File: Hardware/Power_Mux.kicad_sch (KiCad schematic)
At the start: 6 parts, among them U5 TPS2117DRLR

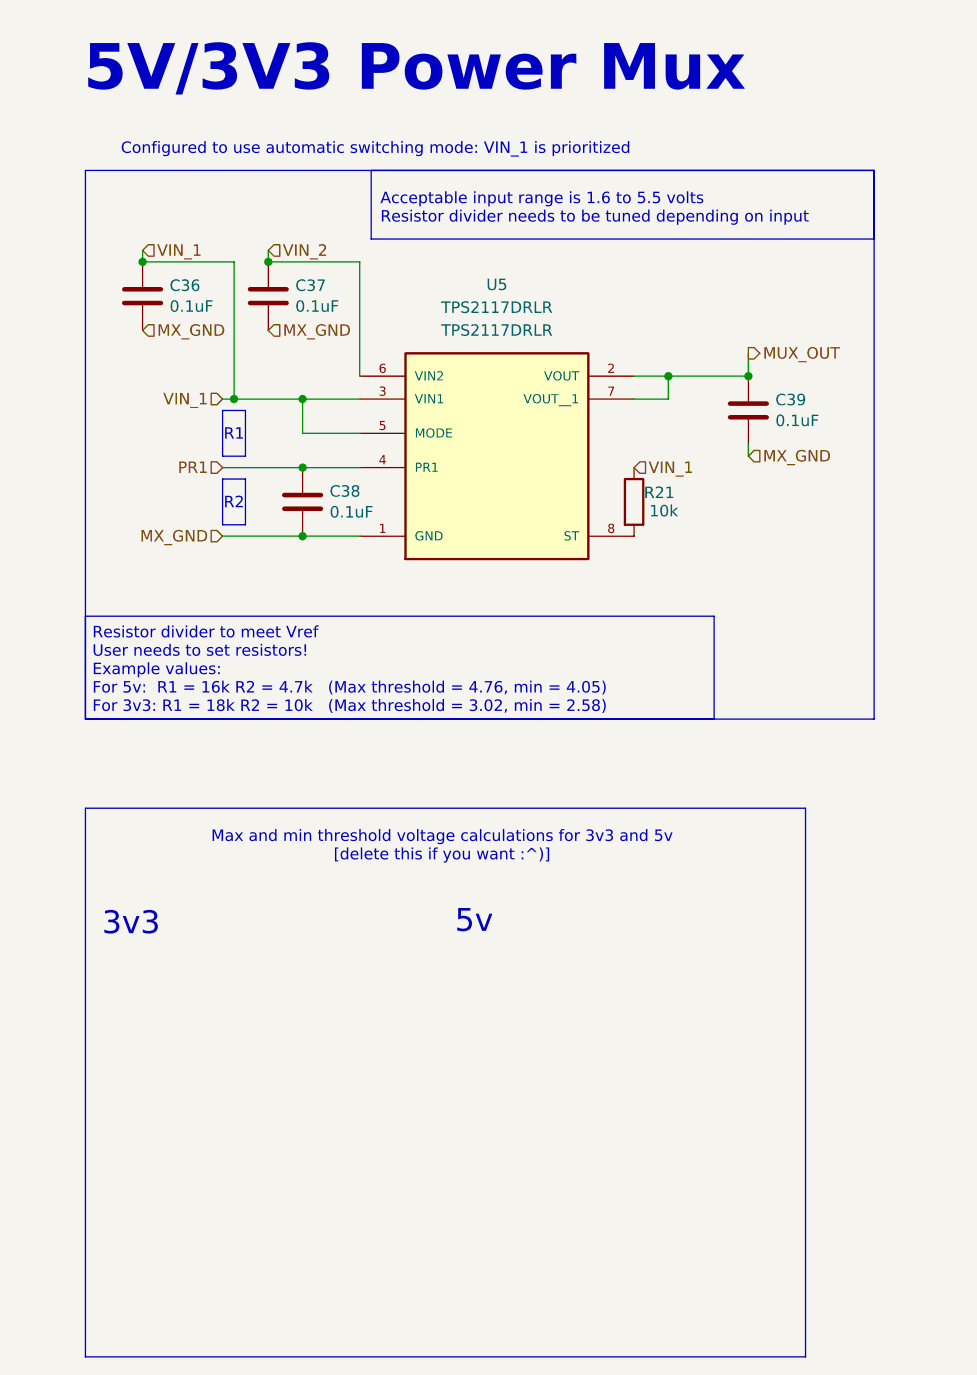
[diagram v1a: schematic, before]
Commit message: made review changes
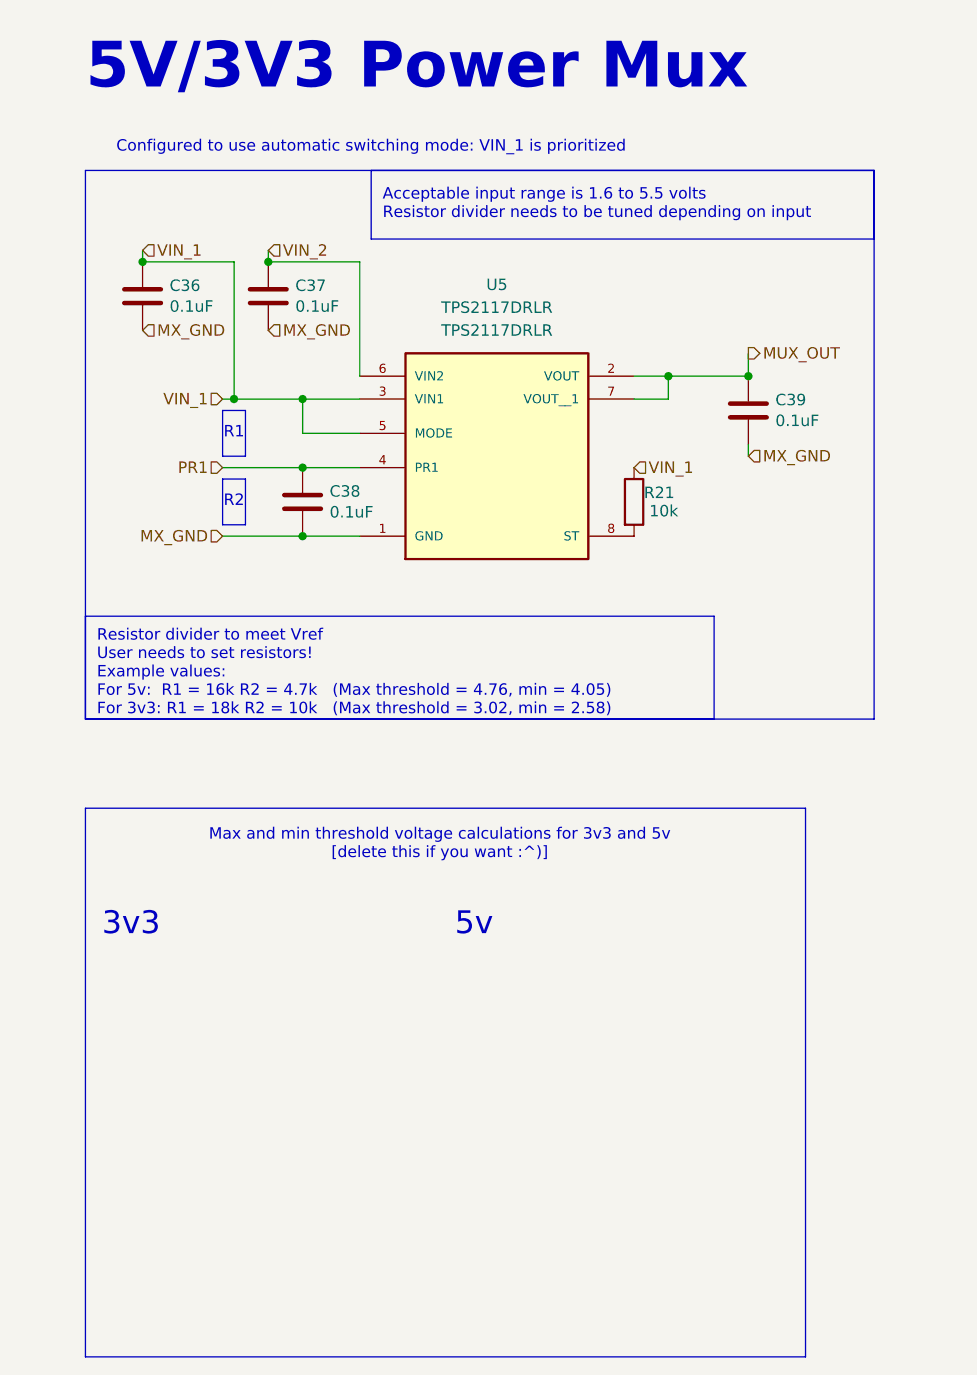
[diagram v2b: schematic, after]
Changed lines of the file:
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@@
 	(text "Max and min threshold voltage calculations for 3v3 and 5v\n[delete this if you want :^)]"
 		(exclude_from_sim no)
-		(at 54.864 106.934 0)
+		(at 54.61 106.68 0)
 		(effects
 			(font
@@
 	(text "R2"
 		(exclude_from_sim no)
-		(at 31.75 68.834 0)
+		(at 31.75 68.58 0)
 		(effects
 			(font
@@
 	(text "R1"
 		(exclude_from_sim no)
-		(at 31.75 61.214 0)
+		(at 31.75 60.96 0)
 		(effects
 			(font
@@
 	(text "5v "
 		(exclude_from_sim no)
-		(at 58.42 115.316 0)
+		(at 58.42 115.57 0)
 		(effects
 			(font
@@
 	(text "Configured to use automatic switching mode: VIN_1 is prioritized"
 		(exclude_from_sim no)
-		(at 47.498 29.464 0)
+		(at 46.99 29.21 0)
 		(effects
 			(font
@@
 	(text "Acceptable input range is 1.6 to 5.5 volts\nResistor divider needs to be tuned depending on input\n"
 		(exclude_from_sim no)
-		(at 48.006 36.068 0)
+		(at 48.26 35.56 0)
 		(effects
 			(font
@@
 	(text "Resistor divider to meet Vref \nUser needs to set resistors!\nExample values:\nFor 5v:  R1 = 16k R2 = 4.7k   (Max threshold = 4.76, min = 4.05)\nFor 3v3: R1 = 18k R2 = 10k   (Max threshold = 3.02, min = 2.58)"
 		(exclude_from_sim no)
-		(at 16.002 87.376 0)
+		(at 16.51 87.63 0)
 		(effects
 			(font
@@
 	(text "5V/3V3 Power Mux"
 		(exclude_from_sim no)
-		(at 51.816 20.574 0)
+		(at 52.07 20.32 0)
 		(effects
 			(font
